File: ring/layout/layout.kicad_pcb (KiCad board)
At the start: 2 copper layers, 62 x 6.2 mm, 62 parts, among them U1 ?, U10 ?, U11 ?, U12 ?, U13 ?, U14 ?, U15 ?, U2 ?, U3 ?, U4 ?, U5 ?, U6 ?, U7 ?, U8 ?, U9 ?, Y1 38.4MHz

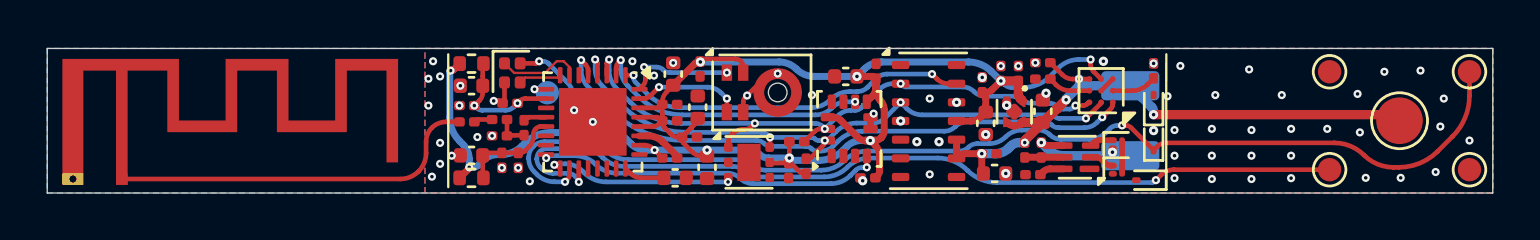
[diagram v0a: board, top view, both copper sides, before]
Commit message: pcb fully fully done
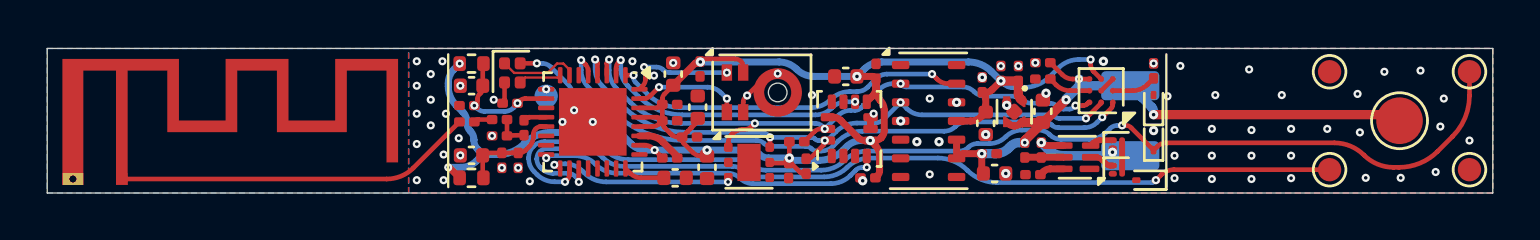
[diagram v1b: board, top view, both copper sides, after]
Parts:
- L2: value 3.2nH -> 3.200000000000001nH
- moved TP1 0.16 mm to (141.2, 82.0)
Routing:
- net VBATT: track 27.8 -> 26.5 mm
- net VDD: track 74.2 -> 75.3 mm
- net GND: track 11.4 -> 10.5 mm, vias 72 -> 77
- net rst: track 1.10 -> 0.30 mm
- net cpu.ant.out3: track 16.1 -> 15.4 mm
